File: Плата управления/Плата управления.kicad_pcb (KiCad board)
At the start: 2 copper layers, 67.6 x 69 mm, 122 parts, among them J1 Conn_01x11, J12 Conn_02x11_Odd_Even, J2 CAN2, J3 CAN1, J4 A, J5 B, J6 C, J7 RS485, U1 AT25xxx, U2 LMV7239M5, U3 LMV324, U4 STM32F767VITx, U5 INA283, U6 ADM3491ExR, U7 ASEMB-10

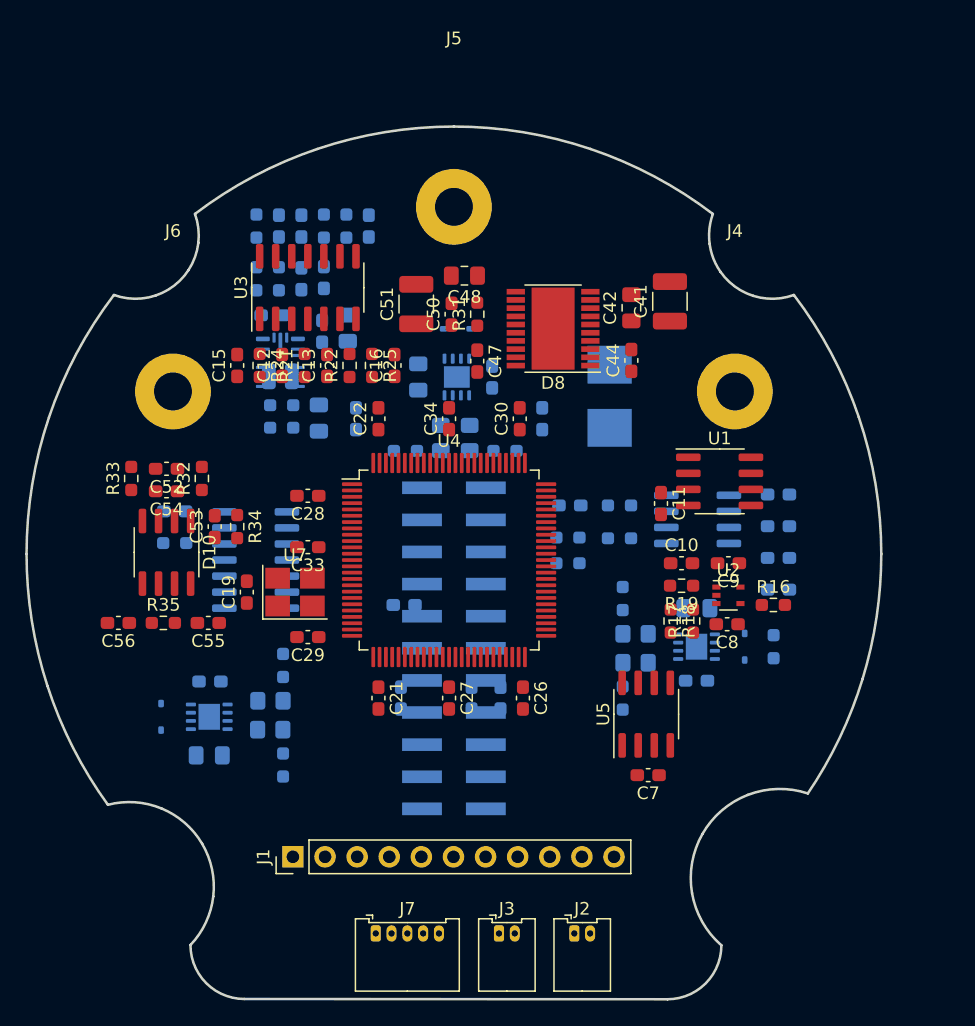
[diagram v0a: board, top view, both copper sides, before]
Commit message: Новый контур платы
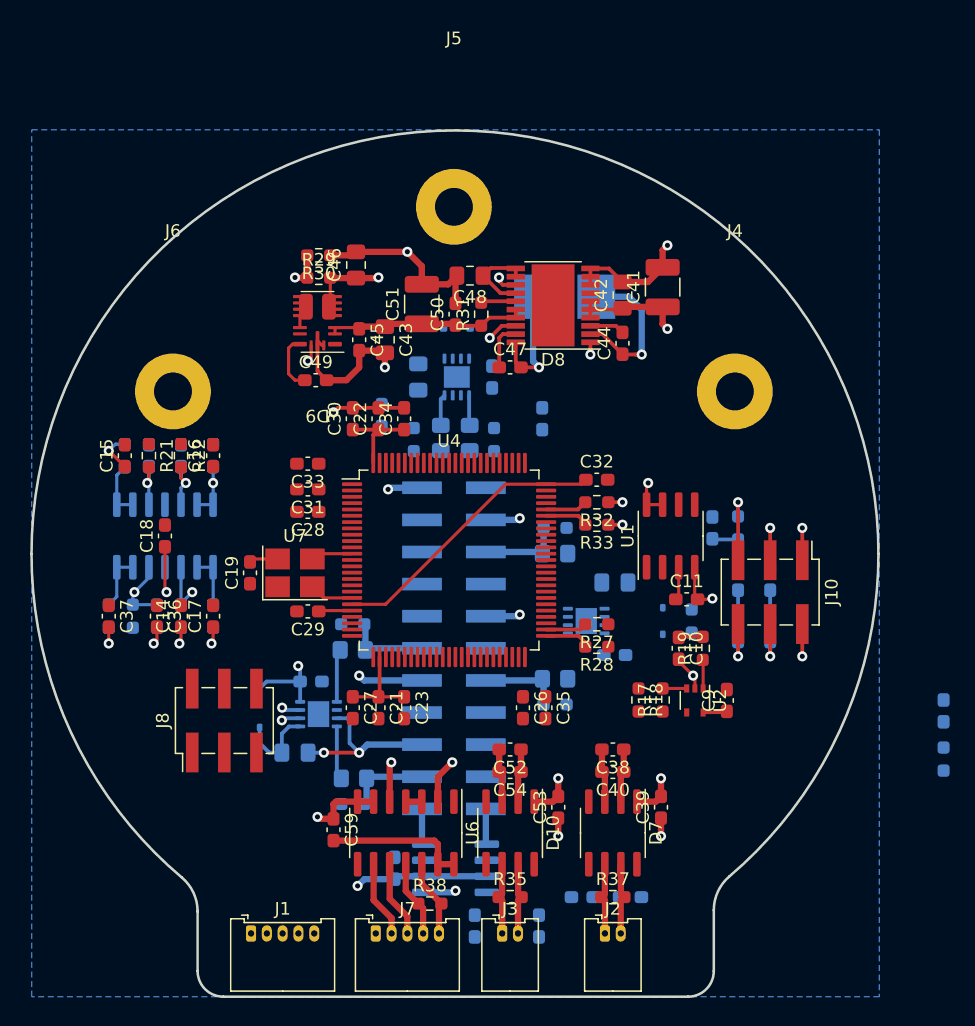
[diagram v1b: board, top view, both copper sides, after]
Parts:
- removed R34, R36: 10k, Resistor_SMD:R_0603_1608Metric_Pad0.98x0.95mm_HandSolder
- added C20: 56p, Capacitor_SMD:C_0603_1608Metric_Pad1.08x0.95mm_HandSolder, B.Cu at (105.7, 98.0)
- added C60: 56p, Capacitor_SMD:C_0603_1608Metric_Pad1.08x0.95mm_HandSolder, B.Cu at (108.2, 98.0)
- added C61: 56p, Capacitor_SMD:C_0603_1608Metric_Pad1.08x0.95mm_HandSolder, B.Cu at (103.6, 94.0)
- added J10: Conn_02x03_Odd_Even, Connector_PinHeader_2.54mm:PinHeader_2x03_P2.54mm_Vertical_SMD, F.Cu at (108.2, 99.1)
- added J8: Conn_02x03_Odd_Even, Connector_PinHeader_2.54mm:PinHeader_2x03_P2.54mm_Vertical_SMD, F.Cu at (65.0, 109.2)
- added R39: 120, Resistor_SMD:R_0603_1608Metric_Pad0.98x0.95mm_HandSolder, B.Cu at (105.7, 102.1)
- added R40: 120, Resistor_SMD:R_0603_1608Metric_Pad0.98x0.95mm_HandSolder, B.Cu at (108.2, 102.1)
- added R41: 120, Resistor_SMD:R_0603_1608Metric_Pad0.98x0.95mm_HandSolder, B.Cu at (105.7, 94.0)
- C12, C13, C55, C56, C7, C8, R16, R24, R25, U3, U5: moved to B.Cu
- C14, C17, C18, C23, C31, C32, C35, C36, C37, C38, C39, C40, C43, C45, C46, C49, C59, D7, D9, R27, R28, R29, R30, R37, R38, U6: moved to F.Cu
- J1: value Conn_01x11 -> RS485; footprint Connector_PinHeader_2.54mm:PinHeader_1x11_P2.54mm_Vertical -> Connector_Molex:Molex_PicoBlade_53048-0510_1x05_P1.25mm_Horizontal
- J12: value Conn_02x11_Odd_Even -> Power
- moved C37 37.1 mm to (55.9, 101.0)
- moved C56 37.0 mm to (84.8, 125.5), turned to 90 degrees
- moved R33 37.0 mm to (94.5, 93.7), turned to 180 degrees
- moved R20 36.1 mm to (55.9, 101.0), turned to -90 degrees
- moved C55 35.5 mm to (89.9, 125.5), turned to -90 degrees
- moved C53 35.1 mm to (91.4, 116.1)
- moved C54 35.1 mm to (87.6, 113.3)
- moved C52 35.1 mm to (87.6, 111.5)
- moved D10 35.1 mm to (87.6, 118.1)
- moved R35 35.0 mm to (87.6, 123.2)
- moved R38 34.9 mm to (81.3, 123.7), turned to 0 degrees
- moved R23 32.9 mm to (61.6, 101.0), turned to 90 degrees
- moved C14 32.3 mm to (61.6, 101.0), turned to 90 degrees
- moved R32 31.3 mm to (94.5, 91.9), turned to 180 degrees
- moved C17 31.3 mm to (64.1, 101.0), turned to 90 degrees
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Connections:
- net Current_C_MCU renamed Digital_input2
- net SCLK_MCU renamed Analog_Input1
- J1 pad 3: GND -> Digital_input1
- J1 pad 4: +3.3V -> Analog_Input2
- U4 pad 51: unconnected-(U4-PB12-Pad51) -> CAN2_RXD_MCU
- U4 pad 52: unconnected-(U4-PB13-Pad52) -> CAN2_TXD_MCU
- U4 pad 70: unconnected-(U4-PA11-Pad70) -> CAN1_RXD_MCU
- U4 pad 71: unconnected-(U4-PA12-Pad71) -> CAN1_TXD_MCU
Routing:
- net GND: track 0.00 -> 84.7 mm, vias 0 -> 17
- net +3.3V: track 0.00 -> 63.6 mm, vias 0 -> 3
- net +12V: track 0.00 -> 23.3 mm, vias 0 -> 1
- net VDDA: track 0.00 -> 22.6 mm
- net C: track 0.00 -> 13.2 mm, vias 0 -> 2
- net Net-(D8-L1): track 0.00 -> 12.8 mm, vias 0 -> 1
- net Temp_C: track 0.00 -> 9.45 mm, vias 0 -> 2
- net Net-(D8-L2): track 0.00 -> 9.36 mm, vias 0 -> 1
- net +24V: track 0.00 -> 9.00 mm, vias 0 -> 1
- net Temp_B: track 0.00 -> 7.42 mm, vias 0 -> 2
- net Temp_A: track 0.00 -> 7.10 mm, vias 0 -> 2
- net Net-(D8-VOS_FB): track 0.00 -> 6.78 mm
- net G6: track 0.00 -> 6.60 mm
- net G1: track 0.00 -> 6.60 mm
- net G2: track 0.00 -> 6.60 mm
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- added copper zone on B.Cu, net GND
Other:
- board size 67.6 x 69 mm -> 67 x 68.5 mm
